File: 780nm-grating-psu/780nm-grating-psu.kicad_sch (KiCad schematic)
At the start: 43 parts, among them Q1 FDD3N40TM, Q2 2N7002, Q3 2N7002, U1 LT3757AEDD

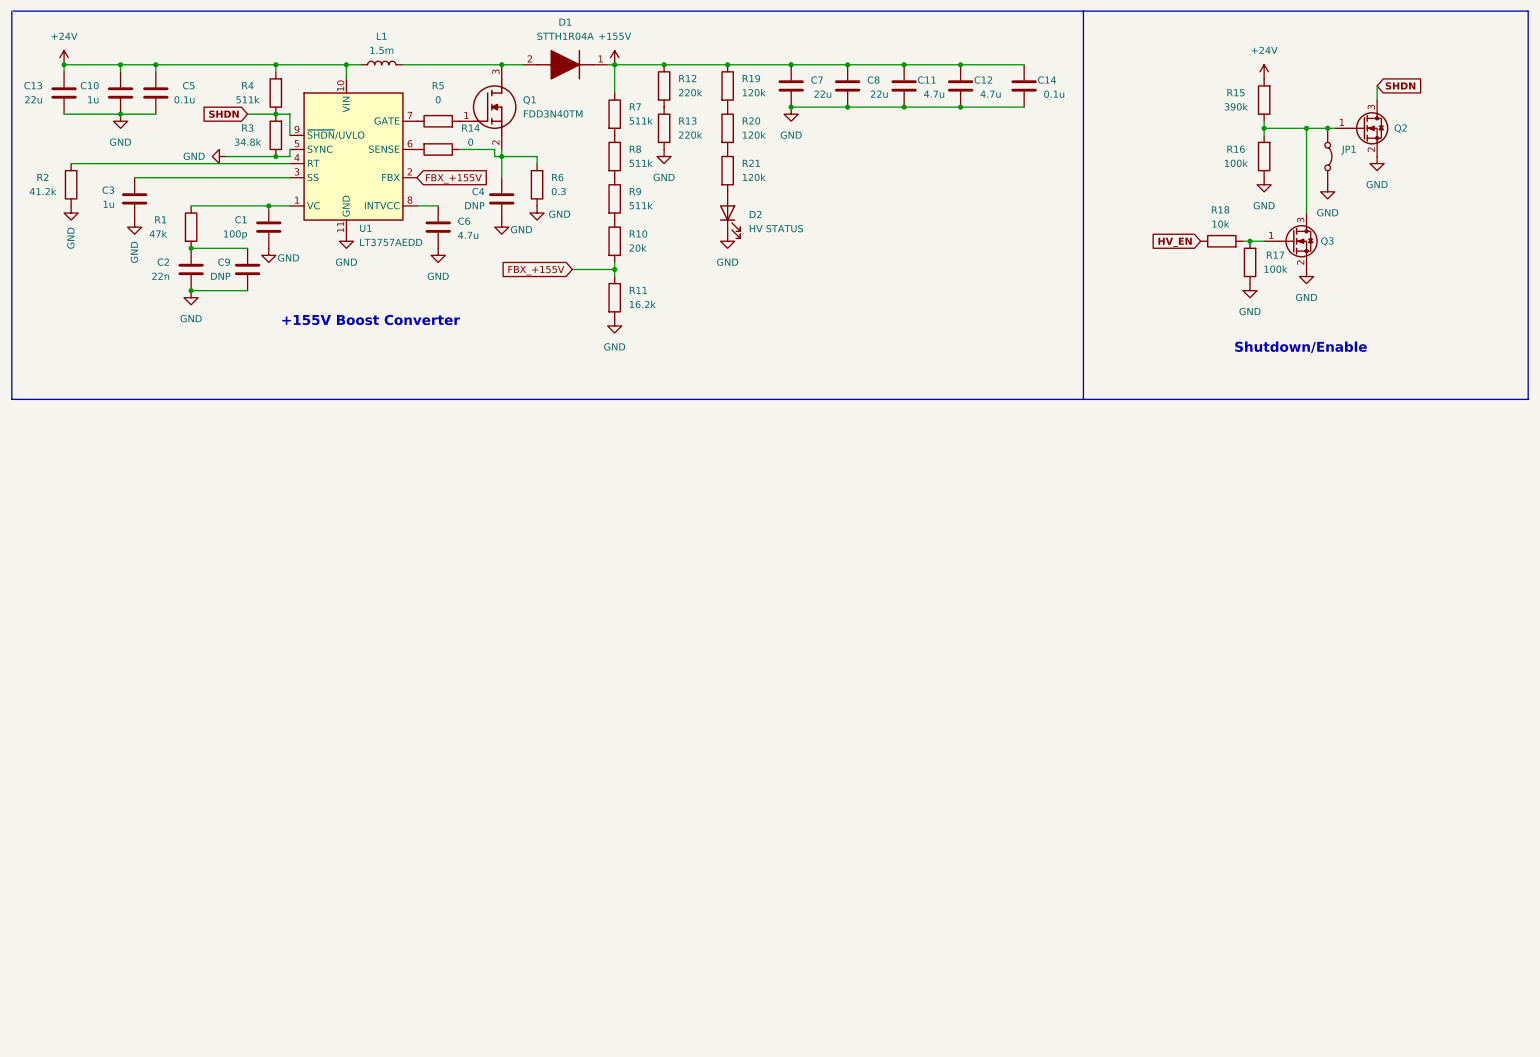
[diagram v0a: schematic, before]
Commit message: psu sch is complete
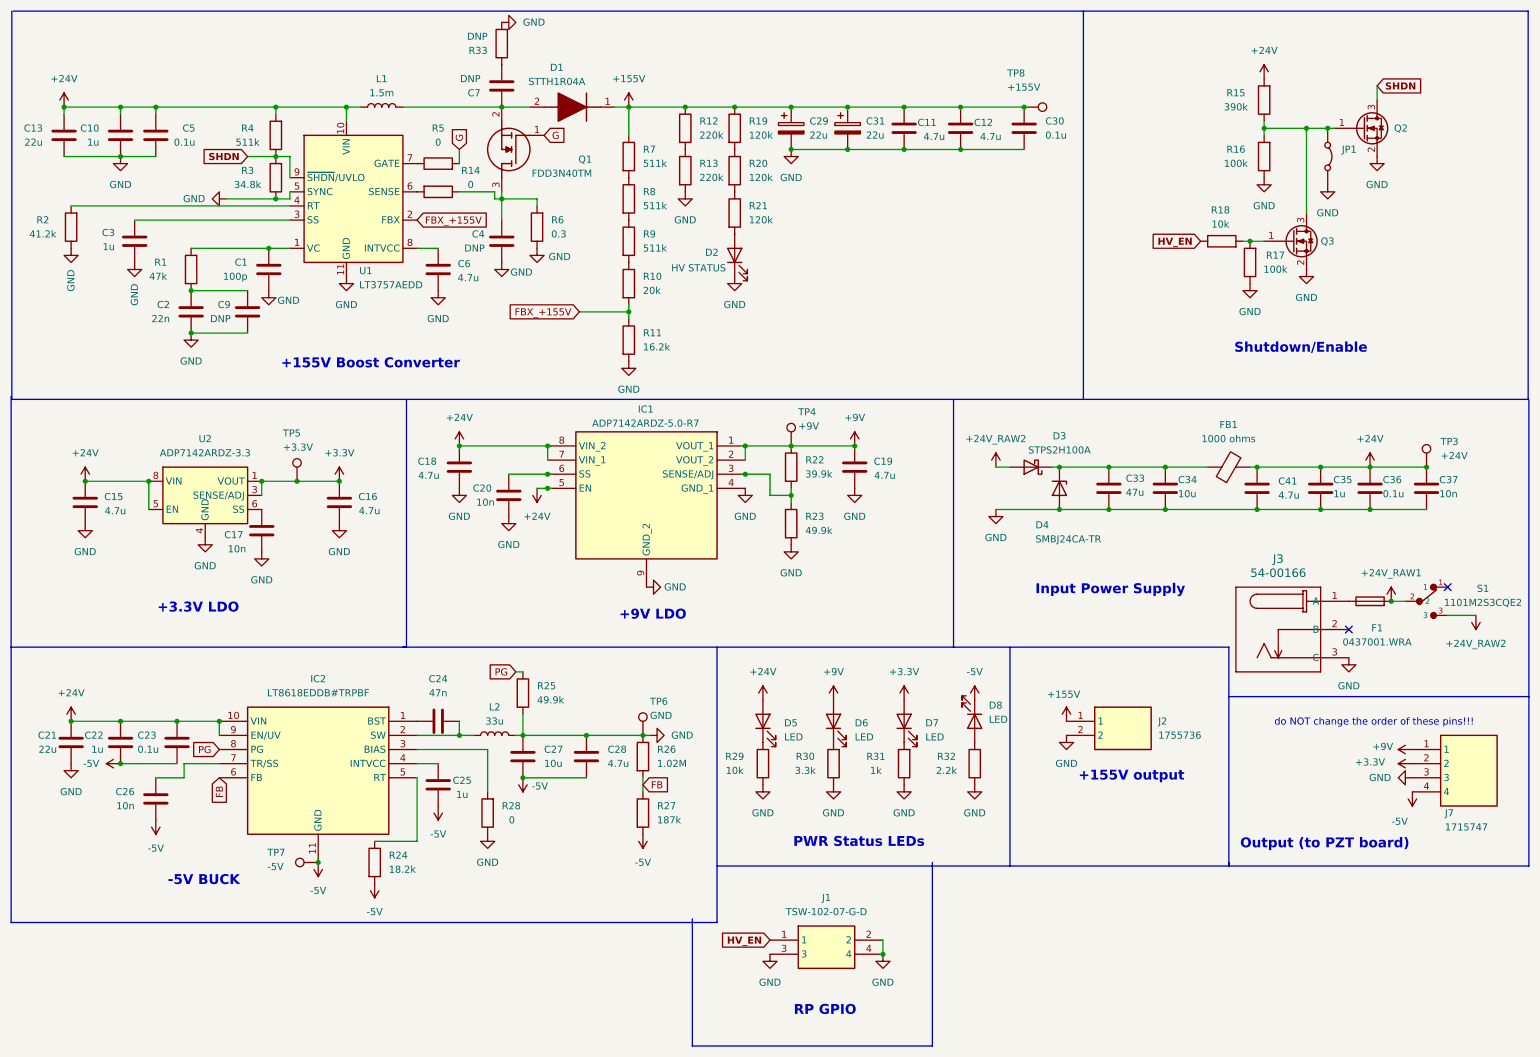
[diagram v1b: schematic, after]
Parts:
- removed C14: 0.1u, Capacitor_SMD:C_0603_1608Metric, symbol Device:C
- removed C8: 22u, Capacitor_SMD:C_0603_1608Metric, symbol Device:C
- added C15, C16, C18, C19, C41: 4.7u, Capacitor_SMD:C_0603_1608Metric, symbol Device:C
- added C17, C26: 10n, Capacitor_SMD:C_0402_1005Metric, symbol Device:C
- added C20, C37: 10n, Capacitor_SMD:C_0603_1608Metric, symbol Device:C
- added C21: 22u, Capacitor_SMD:C_1206_3216Metric, symbol Device:C
- added C22, C25, C35: 1u, Capacitor_SMD:C_0603_1608Metric, symbol Device:C
- added C23, C36: 0.1u, Capacitor_SMD:C_0603_1608Metric, symbol Device:C
- added C24: 47n, Capacitor_SMD:C_0402_1005Metric, symbol Device:C
- added C27: 10u, Capacitor_SMD:C_0402_1005Metric, symbol Device:C
- added C28: 4.7u, Capacitor_SMD:C_0402_1005Metric, symbol Device:C
- added C29, C31: 22u, UCS2E220MPD:PCAP_10x20-THRU-ELECT_NCA, symbol Device:C_Polarized
- added C30: 0.1u, PHE426HA6100JR05:CAP_PHE426_AH_KEM, symbol Device:C
- added C33: 47u, Capacitor_SMD:C_1210_3225Metric, symbol Device:C
- added C34: 10u, Capacitor_SMD:C_0603_1608Metric, symbol Device:C
- added D3: ​​​STPS2H100A, Diode_SMD:D_SMA, symbol Device:D_Schottky
- added D4: SMBJ24CA-TR, Diode_SMD:D_SMB, symbol Diode:PTVS26VZ1USK
- added D5, D6, D7, D8: LED, LED_SMD:LED_0603_1608Metric, symbol Device:LED
- added F1: 0437001.WRA, symbol Device:Fuse
- added FB1: 1000 ohms, Inductor_SMD:L_0603_1608Metric, symbol Device:FerriteBead
- added IC1: ADP7142ARDZ-5.0-R7, SOIC127P600X175-9N, symbol ADP7142ARDZ-R7:ADP7142ARDZ-R7
- added IC2: LT8618EDDB#TRPBF, SON50P200X300X80-11N-D, symbol LT8618EDDB#TRPBF:LT8618EDDB#TRPBF
- added J1: TSW-102-07-G-D, HDRV4W64P254_2X2_508X508X838P, symbol TSW-102-07-G-D:TSW-102-07-G-D
- added J2: 1755736, 1755736:1755736, symbol 1755736:1755736
- added J3: 54-00166, 54-00166:CONN3_54-00166_TEN, symbol 54-00166:54-00166
- added J7: 1715747, 1715747:1715747, symbol 1715747:1715747
- added L2: 33u, symbol Device:L
- added R22: 39.9k, Resistor_SMD:R_0603_1608Metric, symbol Device:R
- added R23, R25: 49.9k, Resistor_SMD:R_0603_1608Metric, symbol Device:R
- added R24: 18.2k, Resistor_SMD:R_0603_1608Metric, symbol Device:R
- added R26: 1.02M, Resistor_SMD:R_0603_1608Metric, symbol Device:R
- added R27: 187k, Resistor_SMD:R_0603_1608Metric, symbol Device:R
- added R28: 0, Resistor_SMD:R_0603_1608Metric, symbol Device:R
- added R29: 10k, Resistor_SMD:R_0603_1608Metric, symbol Device:R
- added R30: 3.3k, Resistor_SMD:R_0603_1608Metric, symbol Device:R
- added R31: 1k, Resistor_SMD:R_0603_1608Metric, symbol Device:R
- added R32: 2.2k, Resistor_SMD:R_0603_1608Metric, symbol Device:R
- added R33: DNP, Resistor_SMD:R_1206_3216Metric, symbol Device:R
- added S1: 1101M2S3CQE2, 1101M2S3CQE2:SW_1101M2S3CQE2, symbol 1101M2S3CQE2:1101M2S3CQE2
- added TP3: +24V, TestPoint:TestPoint_Keystone_5015_Micro_Mini, symbol Connector:TestPoint
- added TP4: +9V, TestPoint:TestPoint_Keystone_5015_Micro_Mini, symbol Connector:TestPoint
- added TP5: +3.3V, TestPoint:TestPoint_Keystone_5015_Micro_Mini, symbol Connector:TestPoint
- added TP6: GND, TestPoint:TestPoint_Keystone_5015_Micro_Mini, symbol Connector:TestPoint
- added TP7: -5V, TestPoint:TestPoint_Keystone_5015_Micro_Mini, symbol Connector:TestPoint
- added TP8: +155V, TestPoint:TestPoint_Pad_D4.0mm, symbol Connector:TestPoint
- added U2: ADP7142ARDZ-3.3, Package_SO:SOIC-8-1EP_3.9x4.9mm_P1.27mm_EP2.29x3mm, symbol Regulator_Linear:ADP7142ARDZ-3.3
- C7: value 22u -> DNP; footprint Capacitor_SMD:C_0603_1608Metric -> Capacitor_SMD:C_1206_3216Metric
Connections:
- net +155V: now also C29.1, C30.1, C31.1, J2.1, TP8.1; no longer C7.2
- net +24V: now also C15.2, C18.2, C21.1, C22.1, C23.1, C35.1, C36.1, C37.1, C41.1, D5.2 (A), FB1.2, IC1.5 (EN), IC1.7 (VIN_1), IC1.8 (VIN_2), IC2.10 (VIN), IC2.9 (EN/UV), TP3.1, U2.5 (EN), U2.7 (VIN), U2.8 (VIN)
- net GND: now also C15.1, C16.1, C17.1, C18.1, C19.1, C20.1, C21.2, C27.2, C28.2, C29.2, C30.2, C31.2, C33.2, C34.2, C35.2, C36.2, C37.2, C41.2, D4.2 (A), IC1.4 (GND_1), IC1.9 (GND_2), J1.2, J1.3, J1.4, J2.2, J3.3 (C), J7.3, L2.2, R23.2, R25.2, R26.1, R28.1, R29.1, R30.1, R31.1, R32.1, R33.2, TP6.1, U2.4 (GND), U2.9 (GND); no longer C7.1
- net HV_EN: now also J1.1
- net G: now reaches Q1.1 (G), R5.2
- net at D1.2 (A), L1.2: now also C7.1, Q1.2 (S); no longer Q1.3 (D)
- net at C4.1, R14.1, R6.2: now also Q1.3 (D); no longer Q1.2 (S)
- new net: C7.2, R33.1
- new net: IC2.3 (BIAS), R28.2
- new net: C24.1, IC2.1 (BST)
- new net: C24.2, IC2.2 (SW), L2.1
- new net: C25.1, IC2.4 (INTVCC)
- new net: D8.2 (A), R32.2
- new net: C33.1, C34.1, D3.1 (K), D4.1 (K), FB1.1
- new net: D7.1 (K), R31.2
- new net: C17.2, U2.6 (SS)
- new net: IC1.3 (SENSE/ADJ), R22.2, R23.1
- new net: IC2.5 (RT), R24.1
- new net: D6.1 (K), R30.2
- new net: C20.2, IC1.6 (SS)
- new net: F1.1, J3.1 (A)
- new net: C26.2, IC2.7 (TR/SS)
- new net: D5.1 (K), R29.2
- new net +24V_RAW1: F1.2, S1.2
- new net +24V_RAW2: D3.2 (A), S1.3
- new net +3.3V: C16.2, D7.2 (A), J7.2, TP5.1, U2.1 (VOUT), U2.2 (VOUT), U2.3 (SENSE/ADJ)
- new net +9V: C19.2, D6.2 (A), IC1.1 (VOUT_1), IC1.2 (VOUT_2), J7.1, R22.1, TP4.1
- new net -5V: C22.2, C23.2, C25.2, C26.1, C27.1, C28.1, D8.1 (K), IC2.11 (GND), J7.4, R24.2, R27.2, TP7.1
- new net FB: IC2.6 (FB), R26.2, R27.1
- new net PG: IC2.8 (PG), R25.1
- no-connect marks 0 -> 2
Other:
- note added: "+155V output"
- note added: "+3.3V LDO"
- note added: "+9V LDO"
- note added: "-5V BUCK"
- note added: "Input Power Supply"
- note added: "Output (to PZT board)"
- note added: "PWR Status LEDs"
- note added: "RP GPIO"
- note added: "do NOT change the order of these pins!!!"
- moved on the sheet: C1, C10, C11, C12, C13, C2, C3, C4, C5, C6, C9, D1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
